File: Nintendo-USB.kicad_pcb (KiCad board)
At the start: 2 copper layers, 27.6 x 19.8 mm, 21 parts, among them J1 USB_A, J2 Conn_02x03_Odd_Even, SW1 SW_Push, U1 ATMEGA32U4, U2 LP5907MFX-3.3, Y1 Crystal

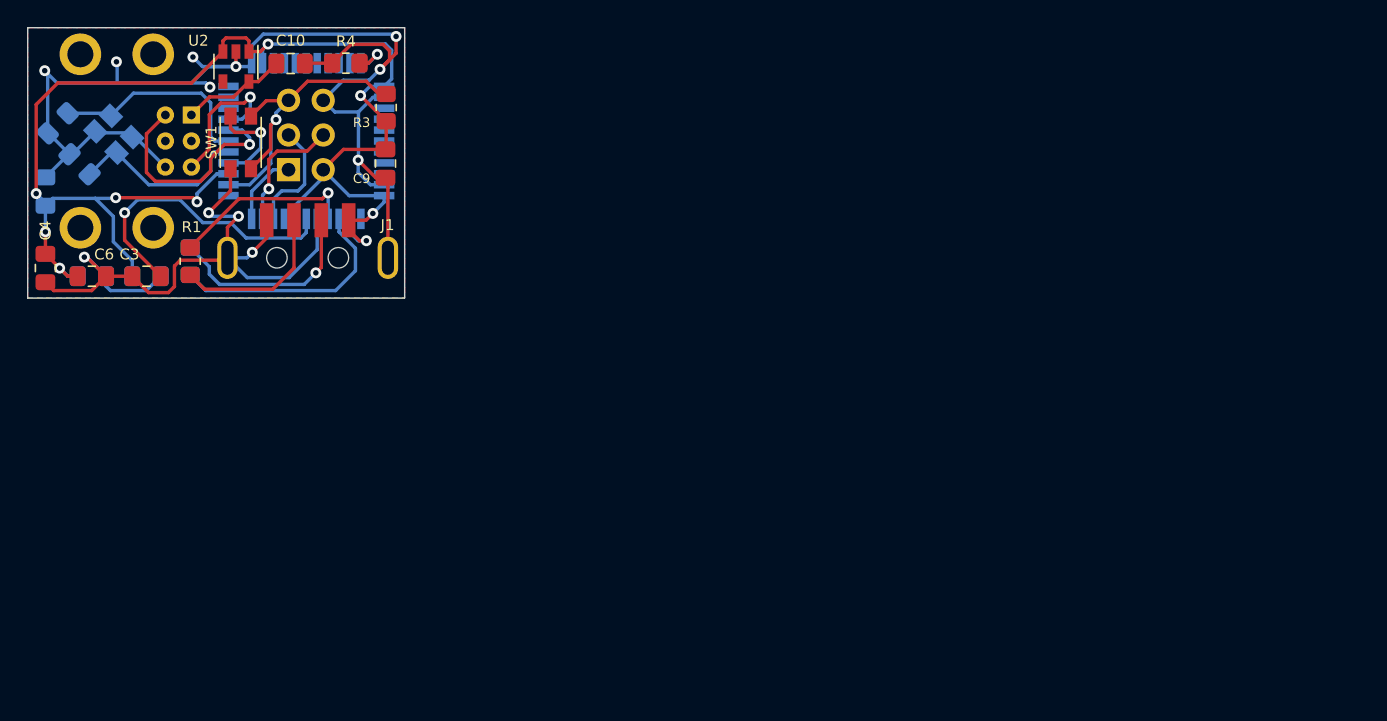
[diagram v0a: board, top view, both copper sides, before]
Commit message: Version 2
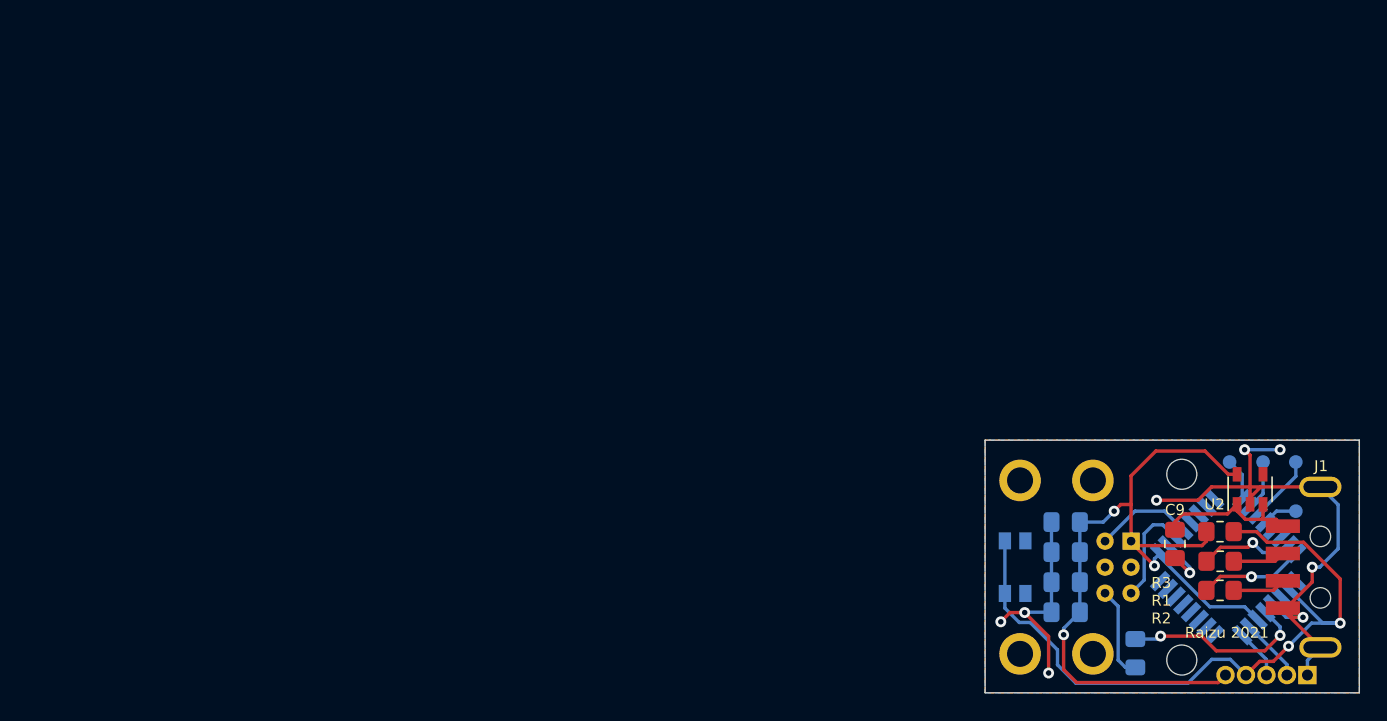
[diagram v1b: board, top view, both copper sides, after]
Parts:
- removed C2: 22pF, Capacitor_SMD:C_0805_2012Metric_Pad1.18x1.45mm_HandSolder
- removed C3: 1uF, Capacitor_SMD:C_0805_2012Metric_Pad1.18x1.45mm_HandSolder
- removed C4, C5: 0.1uF, Capacitor_SMD:C_0805_2012Metric_Pad1.18x1.45mm_HandSolder
- removed J?1: CONN_WII, Raizu_OFFSET:CONN_WII
- removed R4: 10K, Resistor_SMD:R_0805_2012Metric_Pad1.20x1.40mm_HandSolder
- removed Y1: Crystal, Crystal:Crystal_SMD_SeikoEpson_FA238-4Pin_3.2x2.5mm
- added J3: CONN_WII, Raizu_OFFSET:CONN_WII, F.Cu at (181.3, 97.9)
- added REF**: MountingHole_2.2mm_M2, MountingHole:MountingHole_2.2mm_M2, F.Cu at (190.6, 91.1)
- added REF**: MountingHole_2.2mm_M2, MountingHole:MountingHole_2.2mm_M2, F.Cu at (190.6, 104.7)
- added TP1: TestPoint, TestPoint:TestPoint_Pad_D1.0mm, B.Cu at (194.1, 90.2)
- added TP2: TestPoint, TestPoint:TestPoint_Pad_D1.0mm, B.Cu at (196.6, 90.2)
- added TP3: TestPoint, TestPoint:TestPoint_Pad_D1.0mm, B.Cu at (198.9, 90.2)
- added TP4: TestPoint, TestPoint:TestPoint_Pad_D1.0mm, B.Cu at (198.9, 93.8)
- C1: value 22pF -> 1uF
- C10, C6, SW1: moved to B.Cu
- J2: value Conn_02x03_Odd_Even -> Conn_01x05; footprint Connector_PinHeader_2.54mm:PinHeader_2x03_P2.54mm_Vertical -> Connector_PinHeader_2.00mm:PinHeader_1x05_P2.00mm_Vertical; moved to F.Cu
- R2: moved to F.Cu
- U1: value ATMEGA32U4 -> ATSAMD21E15B-A; footprint Package_QFP:TQFP-44_10x10mm_P0.8mm -> Package_QFP:TQFP-32_7x7mm_P0.8mm
- moved C1 87.9 mm to (187.2, 104.2), turned to 270 degrees
- moved J2 80.6 mm to (196.8, 105.8), turned to 270 degrees
- moved U2 80.4 mm to (195.6, 92.2), turned to 90 degrees
- moved R2 79.2 mm to (193.4, 99.6), turned to 0 degrees
- moved R1 78.5 mm to (193.4, 97.5), turned to 180 degrees
- moved J1 76.7 mm to (199.5, 97.9), turned to 90 degrees
- moved C6 75.4 mm to (182.1, 101.2), turned to 0 degrees
- moved U1 74.4 mm to (194.0, 97.9), turned to 45 degrees
- moved C8 74.1 mm to (182.1, 96.8), turned to 0 degrees
- moved C7 70.9 mm to (182.1, 99.0), turned to 0 degrees
- moved R3 68.5 mm to (193.4, 95.3), turned to 0 degrees
- moved C10 65.9 mm to (182.1, 94.6), turned to 180 degrees
- moved SW1 64.7 mm to (178.4, 97.9)
- moved C9 64.2 mm to (190.1, 96.2)
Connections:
- C1 pad 1: GND -> Net-(C1-Pad1)
- C1 pad 2: XTAL_2 -> GND
- C6 pad 2: +5V -> +3V3
- C7 pad 2: +5V -> +3V3
- C8 pad 2: +5V -> +3V3
- J2 pad 1: ICSP_MISO -> GND
- J2 pad 2: +5V -> SWCLK
- J2 pad 3: ICSP_SCK -> SWDIO
- J2 pad 4: ICSP_MOSI -> RESET
- J2 pad 5: RESET -> +3V3
- R1 pad 1: USB_D+ -> Net-(J1-Pad2)
- R1 pad 2: Net-(J1-Pad3) -> USB_D-
- R2 pad 1: Net-(J1-Pad2) -> USB_D+
- R2 pad 2: USB_D- -> Net-(J1-Pad3)
- R3 pad 1: RESET -> +3V3
- R3 pad 2: +5V -> RESET
- U1 pad 10: ICSP_MOSI -> GND
- U1 pad 11: ICSP_MISO -> CON_SDA
- U1 pad 12: Net-(U1-Pad12) -> CON_SCL
- U1 pad 13: RESET -> Net-(U1-Pad13)
- U1 pad 14: +5V -> Net-(U1-Pad14)
- U1 pad 15: GND -> Net-(U1-Pad15)
- U1 pad 16: XTAL_1 -> Net-(U1-Pad16)
- U1 pad 17: XTAL_2 -> Net-(TP1-Pad1)
- U1 pad 18: CON_SCL -> Net-(TP2-Pad1)
- U1 pad 19: CON_SDA -> Net-(TP3-Pad1)
- U1 pad 2: +5V -> Net-(U1-Pad2)
- U1 pad 23: GND -> USB_D-
- U1 pad 24: +5V -> USB_D+
- U1 pad 26: Net-(U1-Pad26) -> RESET
- U1 pad 28: Net-(U1-Pad28) -> GND
- U1 pad 29: Net-(U1-Pad29) -> Net-(C1-Pad1)
- U1 pad 3: USB_D- -> Net-(U1-Pad3)
- U1 pad 30: Net-(U1-Pad30) -> +3V3
- U1 pad 31: Net-(U1-Pad31) -> SWCLK
- U1 pad 32: Net-(U1-Pad32) -> SWDIO
- U1 pad 4: USB_D+ -> Net-(U1-Pad4)
- U1 pad 5: GND -> Net-(U1-Pad5)
- U1 pad 7: +5V -> Net-(U1-Pad7)
- U1 pad 9: ICSP_SCK -> +3V3
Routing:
- net +5V: track 102.4 -> 11.1 mm, vias 9 -> 0
- net GND: track 149.1 -> 69.8 mm, vias 13 -> 9
- net +3V3: track 7.79 -> 61.5 mm, vias 0 -> 3
- net RESET: track 24.9 -> 52.5 mm, vias 1 -> 2
- net Net-(U1-Pad6): track 21.8 -> 0.00 mm, vias 1 -> 0
- net XTAL_2: track 15.4 -> 0.00 mm
- net Net-(C1-Pad1): track 0.00 -> 13.8 mm, vias 0 -> 2
- net XTAL_1: track 13.4 -> 0.00 mm
- net Net-(J1-Pad2): track 15.0 -> 3.83 mm, vias 1 -> 0
- net USB_D-: track 17.5 -> 7.09 mm, vias 0 -> 1
- net CON_SCL: track 16.5 -> 7.21 mm, vias 1 -> 0
- net ICSP_MOSI: track 9.26 -> 0.00 mm, vias 1 -> 0
- net Net-(J1-Pad3): track 12.2 -> 3.89 mm
- net ICSP_SCK: track 8.27 -> 0.00 mm
- net USB_D+: track 13.7 -> 7.73 mm
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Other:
- board size 27.6 x 19.8 mm -> 27.4 x 18.5 mm
- board text added: "C"
- board text added: "D"
- board text added: "G"
- board text added: "R"
- board text added: "Raizu 2021"
- board text added: "V"
